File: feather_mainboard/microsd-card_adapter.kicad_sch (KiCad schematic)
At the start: 10 parts, among them J2 693071020811, J3 61300211121

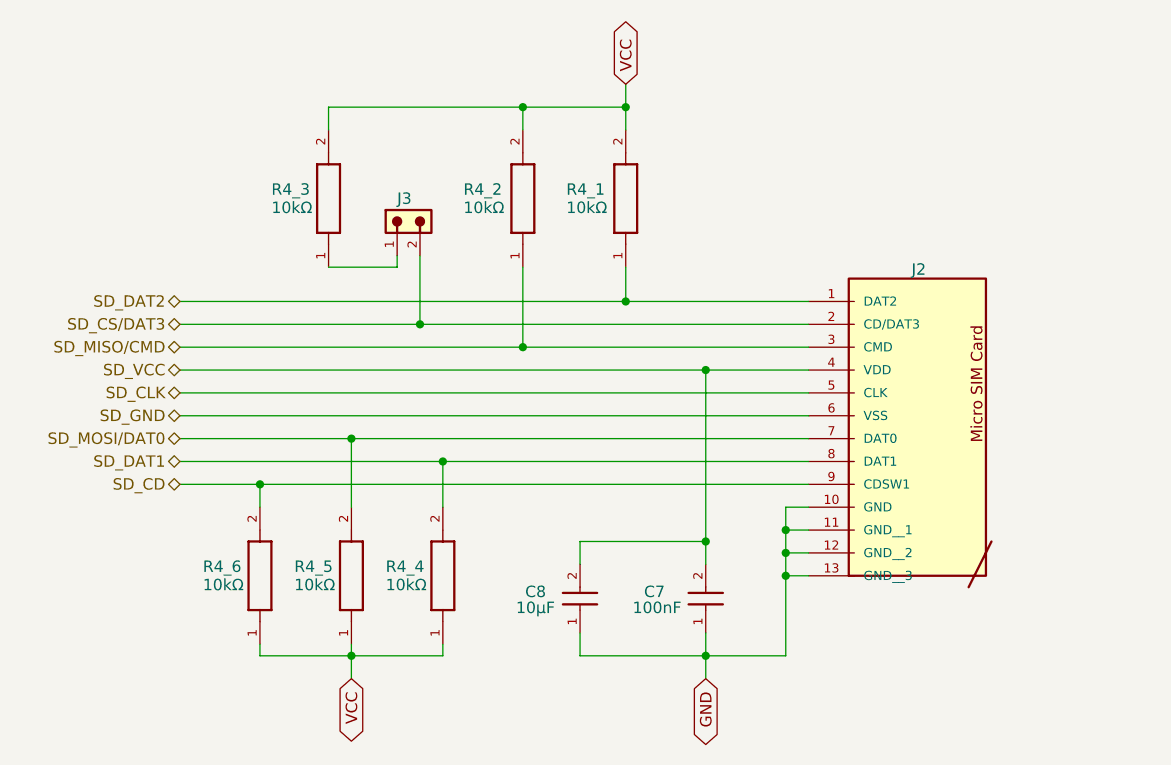
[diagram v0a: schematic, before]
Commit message: finished mainboard design, need to do the routing
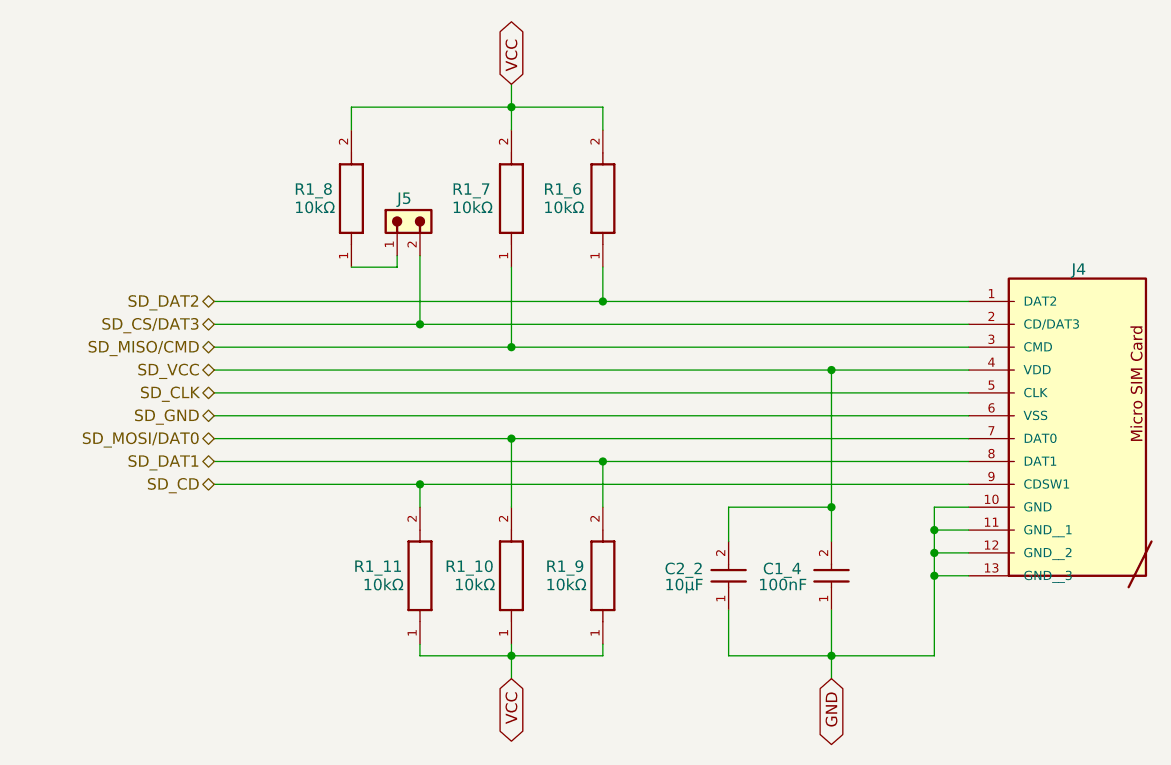
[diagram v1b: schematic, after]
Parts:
- renumbered C7 to C1_4, C8 to C2_2, J2 to J4, J3 to J5, R4_5 to R1_10, R4_6 to R1_11, R4_1 to R1_6, R4_2 to R1_7, R4_3 to R1_8, R4_4 to R1_9
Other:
- moved on the sheet: C1_4, C2_2, J4, R1_10, R1_11, R1_6, R1_7, R1_8, R1_9
